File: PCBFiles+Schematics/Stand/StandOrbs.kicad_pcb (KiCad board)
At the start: 2 copper layers, 50.2 x 23.5 mm, 0 parts

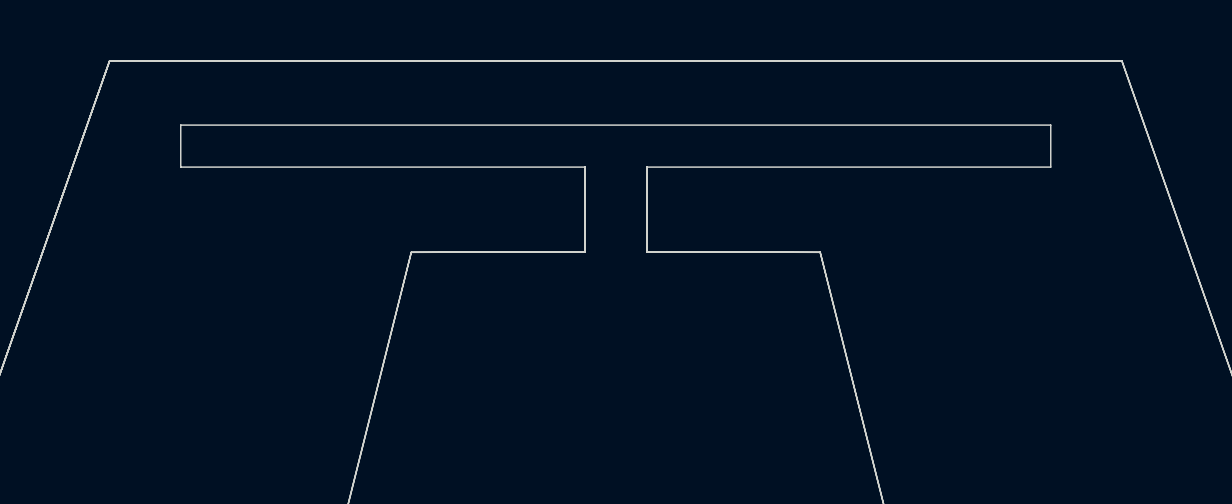
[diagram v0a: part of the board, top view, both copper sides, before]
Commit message: Updated New PCB Files
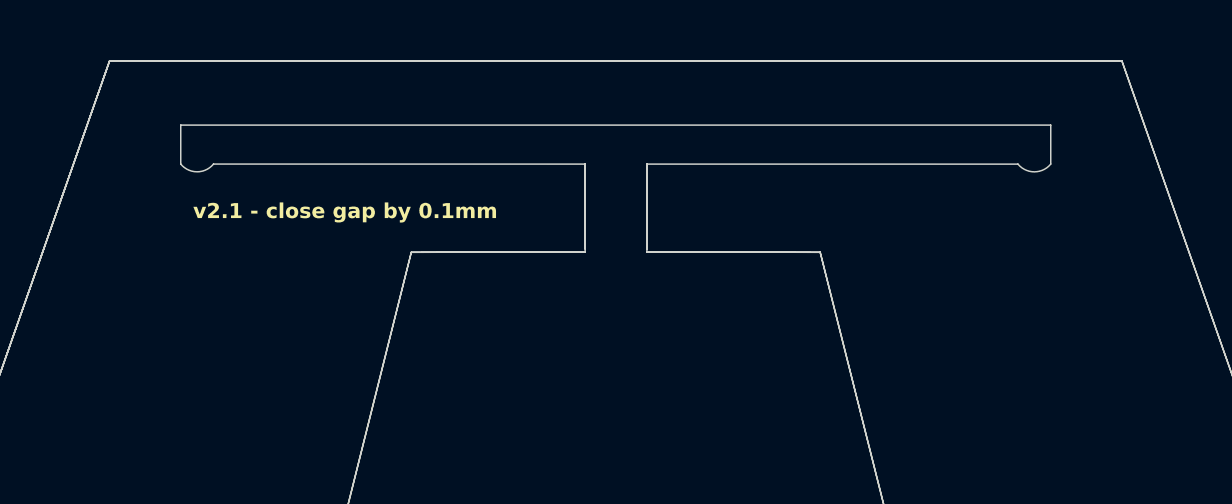
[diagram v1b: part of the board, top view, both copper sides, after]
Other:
- outline, holes or cut-outs redrawn
- board text added: "v2.1 - close gap by 0.1mm"
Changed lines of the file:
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@@
 	)
 	(gr_line
-		(start 98.97 80.44)
+		(start 98.97 80.34)
 		(end 98.97 83.27)
 		(stroke
@@
 	)
 	(gr_line
-		(start 101.03 80.44)
+		(start 101.03 80.34)
 		(end 101.03 83.27)
 		(stroke
@@
 	)
 	(gr_line
-		(start 101.03 83.27)
-		(end 101.03 80.44)
+		(start 101.03 83.17)
+		(end 101.03 80.34)
 		(stroke
 			(width 0.05)
@@
 		(layer "Edge.Cuts")
 	)
+	(gr_arc
+		(start 86.582025 80.338752)
+		(mid 86.036307 80.597081)
+		(end 85.49 80.34)
+		(stroke
+			(width 0.05)
+			(type default)
+		)
+		(layer "Edge.Cuts")
+	)
 	(gr_line
 		(start 125.125 100.44)
@@
 	(gr_line
 		(start 114.49 79.04)
-		(end 114.49 80.44)
+		(end 114.49 80.34)
 		(stroke
 			(width 0.05)
@@
 	(gr_line
 		(start 85.49 79.04)
-		(end 85.49 80.44)
-		(stroke
-			(width 0.05)
-			(type default)
-		)
-		(layer "Edge.Cuts")
-	)
-	(gr_line
-		(start 98.97 80.44)
-		(end 98.97 83.27)
+		(end 85.49 80.34)
+		(stroke
+			(width 0.05)
+			(type default)
+		)
+		(layer "Edge.Cuts")
+	)
+	(gr_line
+		(start 98.97 80.34)
+		(end 98.97 83.17)
 		(stroke
 			(width 0.05)
@@
 	)
 	(gr_line
-		(start 85.49 80.44)
-		(end 98.97 80.44)
+		(start 86.582025 80.338752)
+		(end 98.97 80.34)
 		(stroke
 			(width 0.05)
@@
 	)
 	(gr_line
-		(start 101.03 80.44)
-		(end 114.49 80.44)
+		(start 101.03 80.34)
+		(end 113.397975 80.341248)
 		(stroke
 			(width 0.05)
@@
 		(start 88.875 100.44)
 		(end 74.875 100.44)
+		(stroke
+			(width 0.05)
+			(type default)
+		)
+		(layer "Edge.Cuts")
+	)
+	(gr_arc
+		(start 114.49 80.34)
+		(mid 113.944292 80.598329)
+		(end 113.397975 80.341248)
 		(stroke
 			(width 0.05)
@@
 			)
 			(justify left bottom)
+		)
+	)
+	(gr_text "v2.1 - close gap by 0.1mm"
+		(at 85.9 82.2 0)
+		(layer "F.SilkS")
+		(effects
+			(font
+				(size 0.5 0.5)
+				(thickness 0.125)
+				(bold yes)
+			)
+			(justify left bottom)
